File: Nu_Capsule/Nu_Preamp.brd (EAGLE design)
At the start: 9.4 x 14.8 mm, 20 parts, among them T1 2SC3324, T2 2SC3324

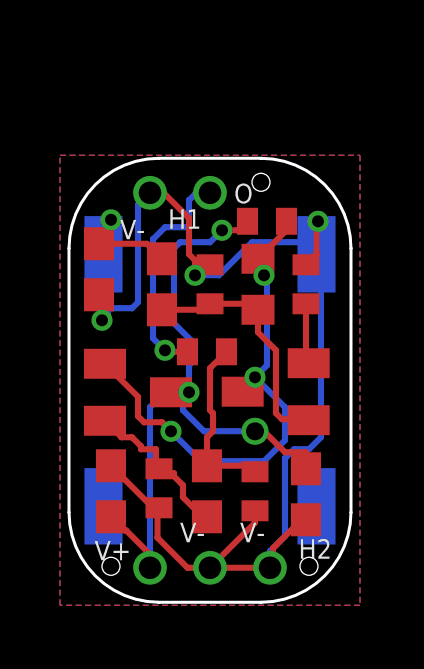
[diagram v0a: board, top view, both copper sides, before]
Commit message: Updated files for version 2.0
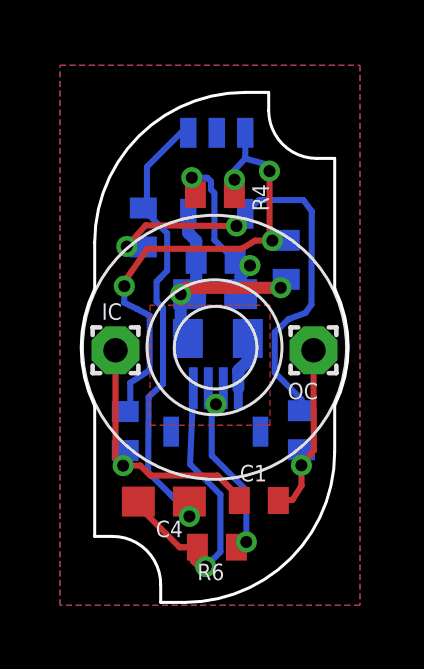
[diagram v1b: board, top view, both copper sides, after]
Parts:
- removed C5: 4.7uF, resistor:C0603
- removed H2: 3P-2MM-TH-MALE, CYCFI_Con:3P-2MM-TH
- removed PAD18, PAD19, PAD6, PAD7: WIREPADSMD1,27-254, wirepad:SMD1,27-2,54
- removed R7: 4.7K, resistor:R0402
- removed T1, T2: 2SC3324, transistor:SOT23
- added D1: (no value), m-pad-2.1:SOD-323
- added IC, OC: (no value), wirepad:1,6/0,8
- added U1: OPA209AIDVBR, CYCFI_semicon:SOT23-5
- C1: value 4.7uF -> 100pF, 25V; device resistor:C0603 -> rcl:C0402
- C2: value 100pF -> 4.7uF, 25V; device resistor:C0603 -> rcl:C0603_NK
- C3: value 4.7uF -> 0.1uF, 25V; device resistor:C0603 -> rcl:C0402
- C4: value 0.1uf -> 4.7uF, 25V; device resistor:C0603 -> rcl:C0603
- H1: value 2P-2MM-TH-MALE -> 4P_ZIF_59453-041110EDHLF; device CYCFI_Con:2P-2MM-TH -> CYCFI_Con:4P_ZIF_59453-041110EDHLF
- R1: value 200K -> 1.2K; device resistor:R0603 -> resistor:R0402
- R2: value 52.3K -> 1.2K
- R3: value 330 -> 22K
- R4: value 22K -> 47K
- R5: value 10K -> 47K
- moved R5 8.72 mm to (7.54, 11.5), flipped to the bottom
- moved C3 8.36 mm to (5.19, 11.5), flipped to the bottom, turned to 0 degrees
- moved H1 8.10 mm to (5.19, 5.74), flipped to the bottom, turned to 0 degrees
- moved C1 7.90 mm to (6.63, 3.49), turned to 0 degrees
- moved R1 6.60 mm to (2.17, 5.81), flipped to the bottom
- moved R3 5.74 mm to (2.78, 12.6), flipped to the bottom, turned to 90 degrees
- moved R2 5.74 mm to (8.05, 5.83), flipped to the bottom, turned to 90 degrees
- moved C2 3.96 mm to (5.17, 10.4), flipped to the bottom, turned to 0 degrees
- moved R6 2.25 mm to (5.23, 1.94), turned to 180 degrees
- moved R4 1.95 mm to (5.16, 13.7)
- moved C4 1.80 mm to (3.46, 3.46), turned to 180 degrees
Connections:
- removed net N$3: C5.2, R5.2, T2.2
- removed net OUTPUT: H1.P$1, R7.2
- removed net VCVF: R1.2, R4.1, T1.3, T2.1
- removed net VIN: C3.2, C4.2, H2.P$1, R4.2, T2.3
- new net N$5: C4.1, R3.2, U1.1
- new net N$6: R1.2, R4.1, R5.2, U1.3
- new net N$7: R2.2, R3.1, U1.4
- new net VCC: C2.2, C3.2, D1.2, R5.1, U1.5
- net GND: now also H1.P$3, R4.2, U1.2; no longer C4.1, H2.P$2, H2.P$3, PAD7.1, R2.1, R3.1, R5.1
- net N$1: now also D1.1, H1.P$1; no longer C1.2, R1.1, R2.2, T1.1
- net N$2: now also IC.1, R1.1; no longer C2.2, PAD6.1
- net N$4: now also C1.2, OC.1, R2.1; no longer R3.2, T1.2
- net OUT: now also C4.2, H1.P$4; no longer C5.1, R7.1
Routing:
- net GND: track 44.2 -> 10.9 mm, vias 3 -> 4
- net VIN: track 24.8 -> 0.00 mm, vias 3 -> 0
- net VCVF: track 17.1 -> 0.00 mm, vias 3 -> 0
- net N$6: track 0.00 -> 16.8 mm, vias 0 -> 4
- net N$5: track 0.00 -> 16.0 mm, vias 0 -> 1
- net N$7: track 0.00 -> 15.6 mm, vias 0 -> 2
- net VCC: track 0.00 -> 9.26 mm, vias 0 -> 2
- net OUTPUT: track 7.71 -> 0.00 mm, vias 1 -> 0
- net N$1: track 8.47 -> 1.80 mm
- net N$3: track 5.40 -> 0.00 mm
- net OUT: track 5.83 -> 10.6 mm, vias 0 -> 1
- net N$4: track 2.02 -> 6.26 mm, vias 0 -> 1
- net N$2: track 4.88 -> 9.05 mm
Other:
- board size 9.4 x 14.8 mm -> 8.9 x 17 mm
- board text removed: "C1"
- board text removed: "C2"
- board text removed: "C3"
- board text removed: "C4"
- board text removed: "C5"
- board text removed: "CYCFI 2016"
- board text removed: "H1"
- board text removed: "H2"
- board text removed: "IC"
- board text removed: "Nu v1.5"
- board text removed: "O"
- board text removed: "OC"
- board text removed: "R1"
- board text removed: "R2"
- board text removed: "R3"
- board text removed: "R4"
- board text removed: "R5"
- board text removed: "R6"
- board text removed: "R7"
- board text removed: "T1"
- board text removed: "T2"
- board text removed: "V+"
- board text removed: "V-"

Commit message: Updated Nu Preamp Files
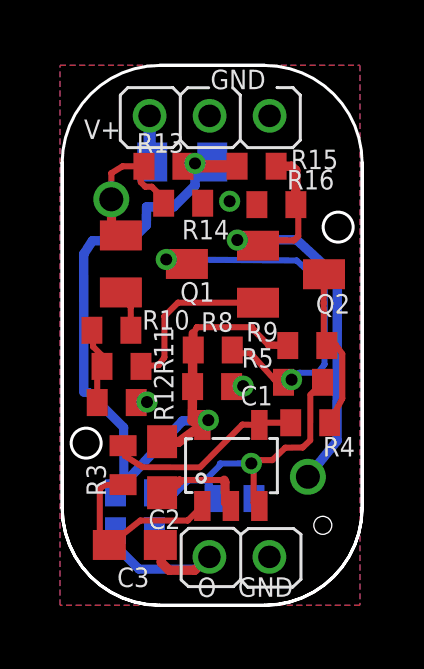
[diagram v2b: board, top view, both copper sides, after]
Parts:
- removed C4: 4.7uF, 25V, rcl:C0603
- removed IC, OC: (no value), wirepad:1,6/0,8
- removed R1: 1.2K, resistor:R0402
- added H2: 3P-2MM-TH-MALE, CYCFI_Con:3P-2MM-TH
- added Q1, Q2: 2SC3324, CYCFI_semicon:SOT23
- added R10, R11: 1.2k, rcl:R0402
- added R12: 12k, rcl:R0402
- added R13, R15: 100k, rcl:R0402
- added R14, R16: 51k, rcl:R0402
- added R7: 150k, resistor:R0402
- added R8, R9: 33k, rcl:R0402
- C1: value 100pF, 25V -> 0.1uF, 25V
- C3: value 0.1uF, 25V -> 10uF, 25V; device rcl:C0402 -> rcl:C0603_NK
- H1: value 4P_ZIF_59453-041110EDHLF -> 2P-2MM-TH-MALE; device CYCFI_Con:4P_ZIF_59453-041110EDHLF -> CYCFI_Con:2P-2MM-TH
- R2: value 1.2K -> 10k; device resistor:R0402 -> rcl:R0402
- R3: value 22K -> 75k
- R4, R5: value 47K -> 33k
- R6: value 10K -> 150k
- U1: value OPA209AIDVBR -> TLV170
- moved C3 9.86 mm to (2.50, 2.01), flipped to the top
- moved U1 9.75 mm to (5.70, 4.66), flipped to the top, turned to 0 degrees
- moved R4 8.24 mm to (8.34, 6.08)
- moved R3 7.95 mm to (2.10, 4.67), flipped to the top
- moved R2 6.48 mm to (2.50, 2.48), turned to 0 degrees
- moved C2 6.03 mm to (3.40, 4.60), flipped to the top, turned to 90 degrees
- moved D1 6.00 mm to (4.08, 14.8), turned to 180 degrees
- moved H1 4.20 mm to (5.98, 1.61), flipped to the top
- moved R5 4.12 mm to (8.10, 7.43), flipped to the top, turned to 0 degrees
- moved C1 4.10 mm to (5.07, 7.29)
- moved R6 1.72 mm to (5.82, 3.56), flipped to the bottom
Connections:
- removed net N$2: C1.1, IC.1, R1.1
- removed net N$4: C1.2, OC.1, R2.1
- removed net N$7: R2.2, R3.1, U1.4
- removed net OUT: C4.2, H1.P$4, R6.2
- removed net VCC: C2.2, C3.2, D1.2, R5.1, U1.5
- new net IN+: Q1.1, R13.1, R14.2
- new net IN-: Q2.1, R15.1, R16.2
- new net N$10: Q2.2, R11.2
- new net N$13: R10.1, R11.1, R12.2
- new net N$14: R5.2, R6.1, R7.2, U1.3
- new net N$15: R3.2, R4.2, U1.4
- new net N$16: C3.1, R3.1, U1.1
- new net N$19: D1.1, H2.P$1
- new net N$9: Q1.2, R10.2
- new net VCC1: C1.1, C2.2, D1.2, R13.2, R15.2, R7.1, R8.2, R9.2, U1.5
- net GND: now also C1.2, H2.P$2, H2.P$3, R12.1, R14.1, R16.1, R2.1, R6.2; no longer C3.1, H1.P$3, R4.2, R6.1
- net N$1: now also C3.2, R2.2; no longer D1.1
- net N$5: now also Q1.3, R5.1, R8.1; no longer C4.1, R3.2, U1.1
- net N$6: now also Q2.3, R9.1; no longer R1.2, R5.2, U1.3
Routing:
- net VCC1: track 0.00 -> 30.6 mm, vias 0 -> 2
- net IN-: track 0.00 -> 16.1 mm, vias 0 -> 2
- net N$7: track 15.6 -> 0.00 mm, vias 2 -> 0
- net N$6: track 16.8 -> 5.47 mm, vias 4 -> 0
- net OUT: track 10.6 -> 0.00 mm, vias 1 -> 0
- net N$14: track 0.00 -> 10.3 mm, vias 0 -> 1
- net VCC: track 9.26 -> 0.00 mm, vias 2 -> 0
- net N$2: track 9.05 -> 0.00 mm, vias 1 -> 0
- net GND: track 10.9 -> 3.36 mm, vias 4 -> 3
- net N$15: track 0.00 -> 6.91 mm
- net N$16: track 0.00 -> 6.42 mm
- net N$4: track 6.26 -> 0.00 mm, vias 1 -> 0
- net N$10: track 0.00 -> 5.59 mm
- net IN+: track 0.00 -> 5.12 mm, vias 0 -> 1
- net N$1: track 1.80 -> 6.57 mm
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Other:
- board size 8.9 x 17 mm -> 10 x 18 mm
- board text added: "GND"
- board text added: "O"
- board text added: "V+"
